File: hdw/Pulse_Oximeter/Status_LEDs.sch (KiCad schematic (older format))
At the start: 20 parts

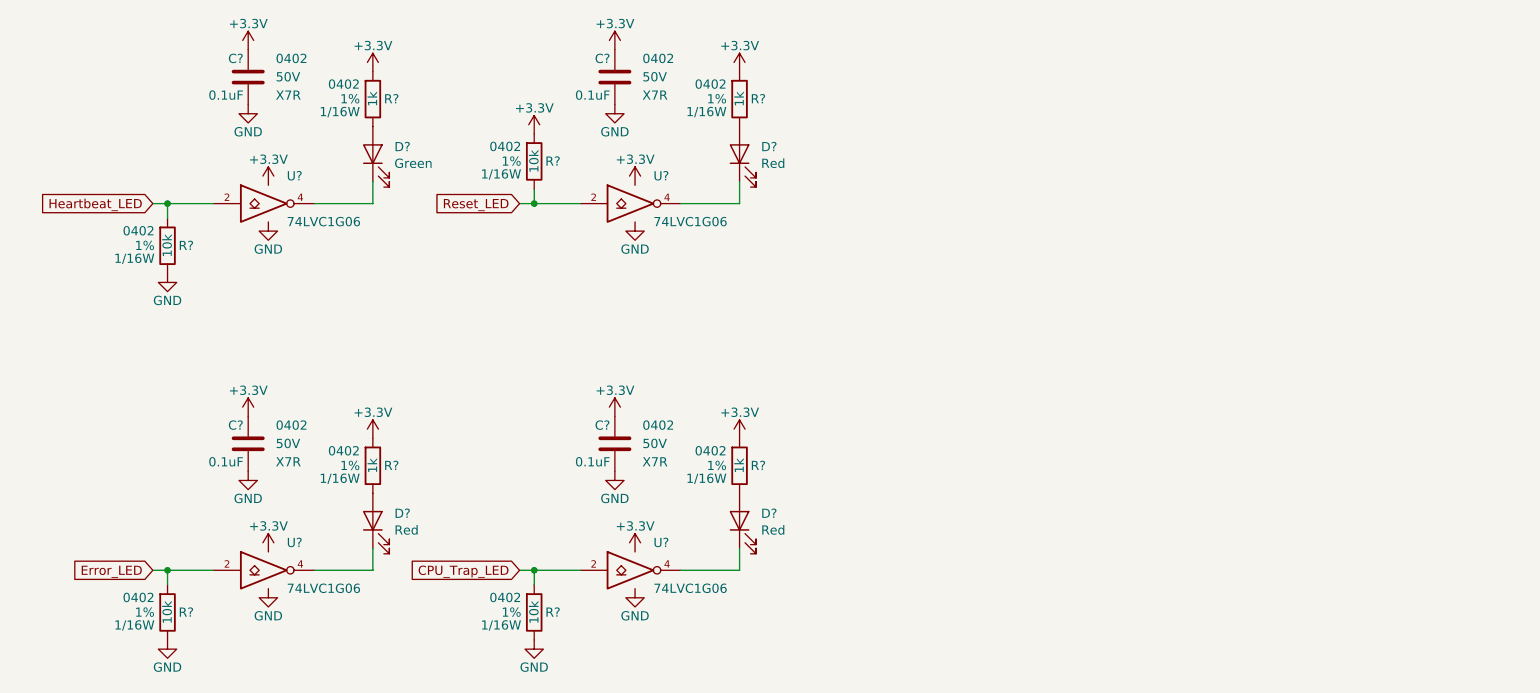
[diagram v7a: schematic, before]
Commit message: Added digikey pn's, footprints
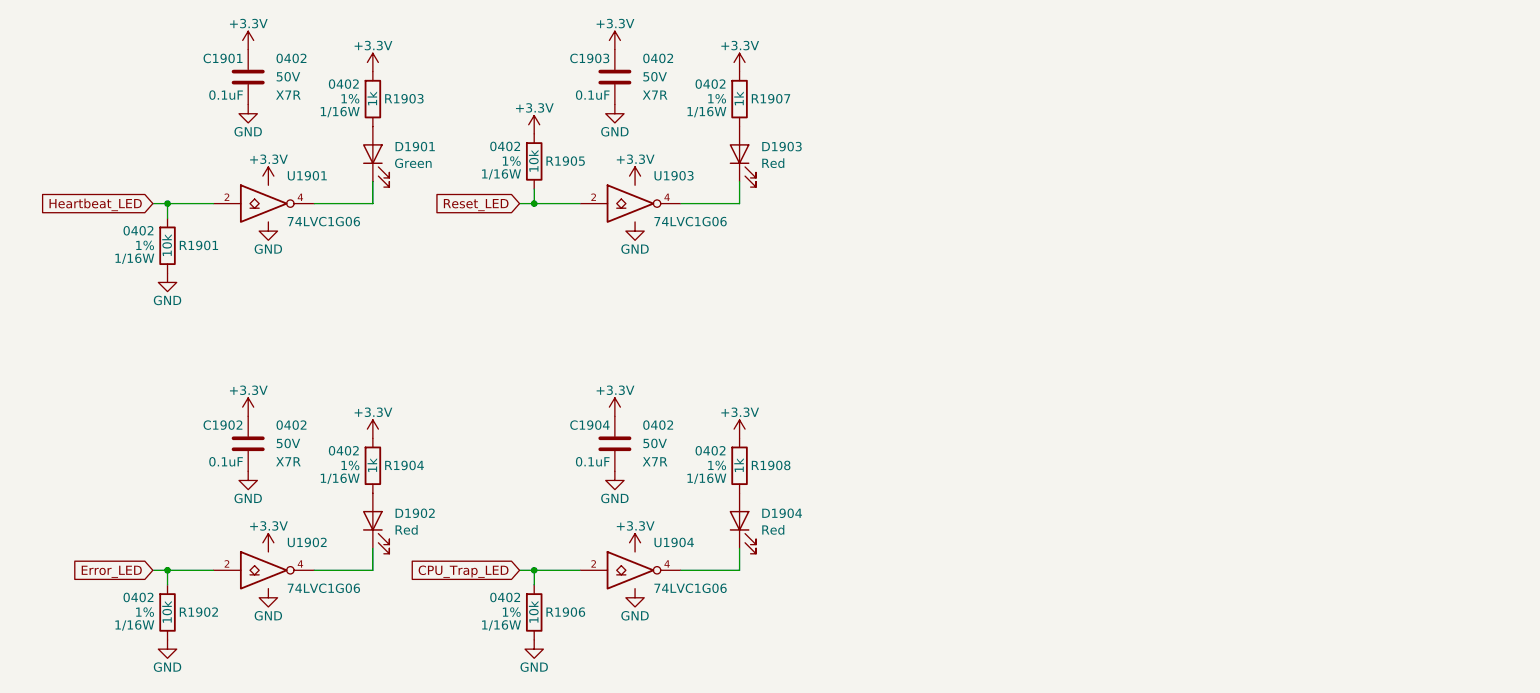
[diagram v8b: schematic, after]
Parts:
- gave numbers to parts that had none: 20
